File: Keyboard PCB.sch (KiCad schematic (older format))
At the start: 150 parts, among them SW1 SW_Push, U1 ATmega32U4-AU, Y1 16MHz

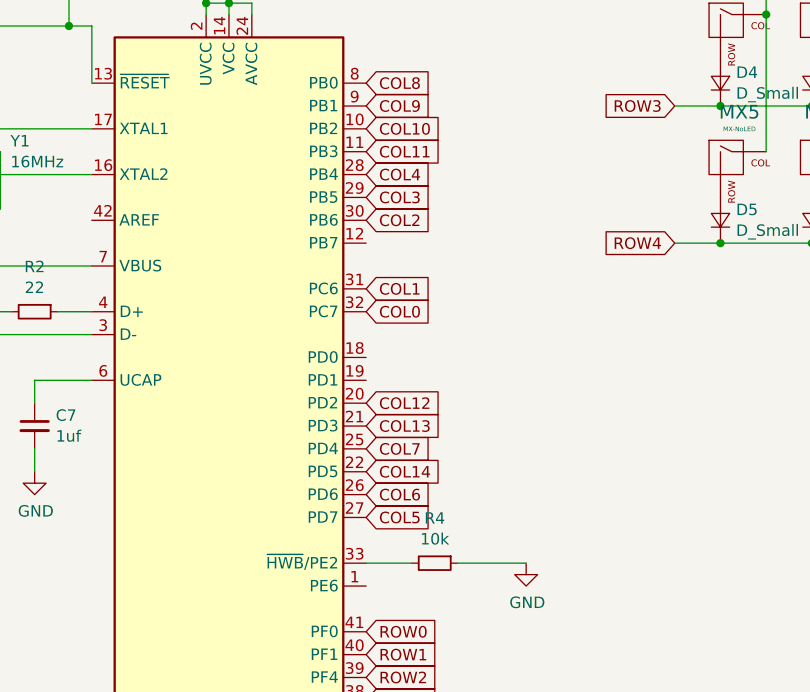
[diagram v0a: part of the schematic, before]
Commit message: fixes
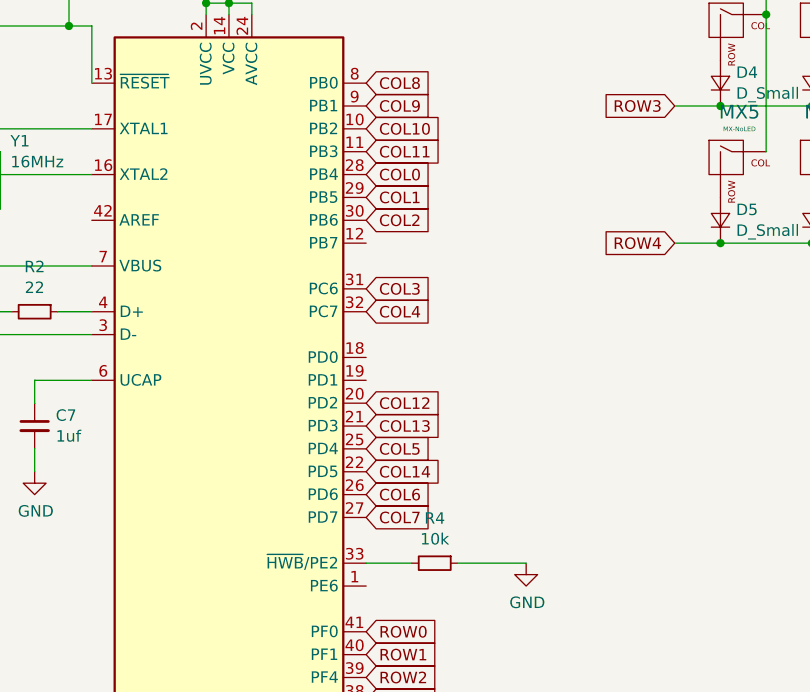
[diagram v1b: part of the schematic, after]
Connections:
- net COL0: now also U1.28 (PB4); no longer U1.32 (PC7)
- net COL1: now also U1.29 (PB5); no longer U1.31 (PC6)
- net COL3: now also U1.31 (PC6); no longer U1.29 (PB5)
- net COL4: now also U1.32 (PC7); no longer U1.28 (PB4)
- net COL5: now also U1.25 (PD4); no longer U1.27 (PD7)
- net COL7: now also U1.27 (PD7); no longer U1.25 (PD4)
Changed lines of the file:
@@
 Text GLabel 3100 3700 2    50   Input ~ 0
 COL8
-Text GLabel 3100 5300 2    50   Input ~ 0
+Text GLabel 3100 5600 2    50   Input ~ 0
 COL7
 Text GLabel 3100 5500 2    50   Input ~ 0
 COL6
-Text GLabel 3100 5600 2    50   Input ~ 0
+Text GLabel 3100 5300 2    50   Input ~ 0
 COL5
-Text GLabel 3100 4700 2    50   Input ~ 0
+Text GLabel 3100 4100 2    50   Input ~ 0
 COL0
-Text GLabel 3100 4600 2    50   Input ~ 0
+Text GLabel 3100 4200 2    50   Input ~ 0
 COL1
 Text GLabel 3100 4300 2    50   Input ~ 0
 COL2
-Text GLabel 3100 4200 2    50   Input ~ 0
+Text GLabel 3100 4600 2    50   Input ~ 0
 COL3
-Text GLabel 3100 4100 2    50   Input ~ 0
+Text GLabel 3100 4700 2    50   Input ~ 0
 COL4
 $EndSCHEMATC
